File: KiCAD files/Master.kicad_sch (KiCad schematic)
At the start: 24 parts, among them SW1 EG1271A, SW2 EG1271A, SW3 EG1271A, SW4 EG1271A, U4 NUCLEO64-F446RE

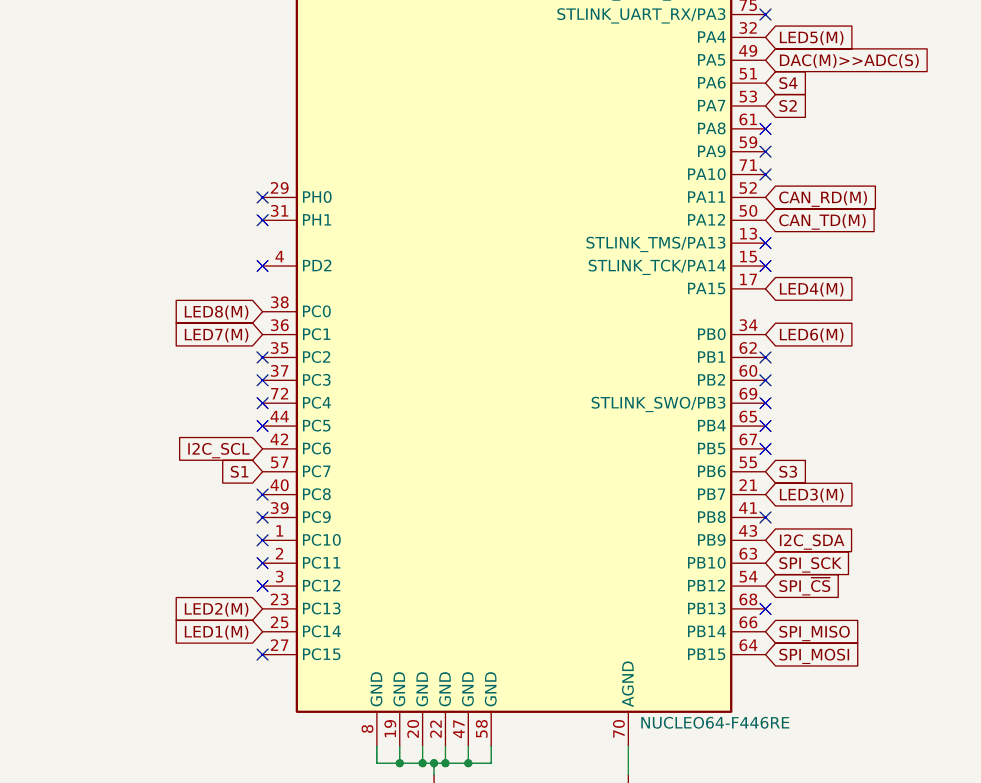
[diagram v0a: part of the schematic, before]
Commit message: update
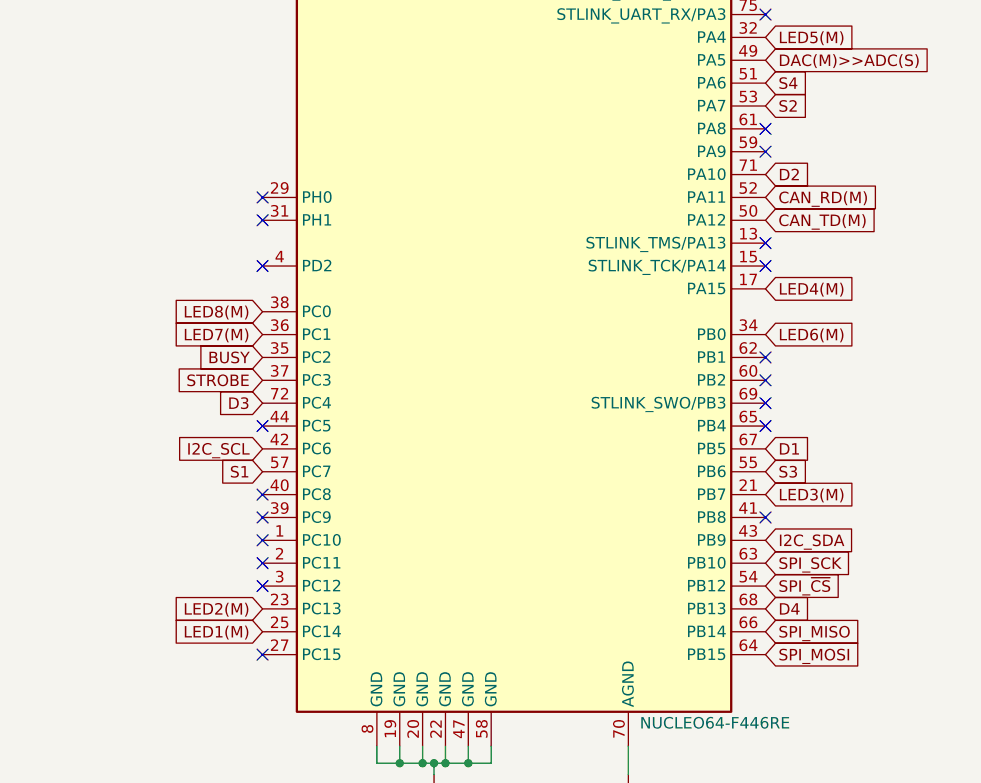
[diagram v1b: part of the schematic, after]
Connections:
- net BUSY: now reaches U4.35 (PC2)
- net STROBE: now reaches U4.37 (PC3)
- net D1: now reaches U4.67 (PB5)
- net D4: now reaches U4.68 (PB13)
- net D2: now reaches U4.71 (PA10)
- net D3: now reaches U4.72 (PC4)
- no-connect marks 40 -> 34
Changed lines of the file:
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@@
   )
   (no_connect (at 169.545 73.66))
-  (no_connect (at 113.665 101.6))
+  (no_connect (at 169.545 106.68))
   (no_connect (at 57.785 136.525))
   (no_connect (at 113.665 53.34))
-  (no_connect (at 169.545 76.2))
   (no_connect (at 113.665 116.84))
   (no_connect (at 113.665 106.68))
@@
   (no_connect (at 169.545 116.84))
   (no_connect (at 113.665 83.82))
-  (no_connect (at 113.665 99.06))
-  (no_connect (at 113.665 104.14))
   (no_connect (at 169.545 88.9))
   (no_connect (at 57.785 147.32))
@@
   (no_connect (at 169.545 104.14))
   (no_connect (at 139.065 40.64))
-  (no_connect (at 169.545 106.68))
   (no_connect (at 58.42 125.73))
   (no_connect (at 169.545 60.96))
@@
   (no_connect (at 144.145 40.64))
   (no_connect (at 131.445 40.64))
-  (no_connect (at 169.545 78.74))
   (no_connect (at 169.545 101.6))
   (no_connect (at 169.545 58.42))
@@
   (no_connect (at 128.905 40.64))
   (no_connect (at 113.665 88.9))
-  (no_connect (at 169.545 127))
+  (no_connect (at 169.545 99.06))
   (no_connect (at 113.665 132.08))
-  (no_connect (at 169.545 99.06))
+  (no_connect (at 169.545 76.2))
   (no_connect (at 126.365 40.64))
   (no_connect (at 169.545 86.36))
   (no_connect (at 113.665 114.3))
-  (no_connect (at 169.545 109.22))
   (no_connect (at 141.605 40.64))
   (wire (pts (xy 39.37 43.18) (xy 39.37 43.815))
@@
     )
   )
+  (global_label "D4" (shape input) (at 169.545 127 0) (fields_autoplaced)
+    (effects (font (size 1.27 1.27)) (justify left))
+    (property "Intersheetrefs" "${INTERSHEET_REFS}" (at 175.0097 127 0)
+      (effects (font (size 1.27 1.27)) (justify left) hide)
+    )
+  )
   (global_label "SPI_MISO" (shape input) (at 140.97 168.91 270) (fields_autoplaced)
     (effects (font (size 1.27 1.27)) (justify right))
@@
     )
   )
+  (global_label "D2" (shape input) (at 169.545 78.74 0) (fields_autoplaced)
+    (effects (font (size 1.27 1.27)) (justify left))
+    (property "Intersheetrefs" "${INTERSHEET_REFS}" (at 175.0097 78.74 0)
+      (effects (font (size 1.27 1.27)) (justify left) hide)
+    )
+  )
   (global_label "LED2(M)" (shape input) (at 29.845 38.1 90) (fields_autoplaced)
     (effects (font (size 1.27 1.27)) (justify left))
@@
     )
   )
+  (global_label "D3" (shape input) (at 113.665 104.14 180) (fields_autoplaced)
+    (effects (font (size 1.27 1.27)) (justify right))
+    (property "Intersheetrefs" "${INTERSHEET_REFS}" (at 108.2003 104.14 0)
+      (effects (font (size 1.27 1.27)) (justify right) hide)
+    )
+  )
   (global_label "S2" (shape input) (at 169.545 71.12 0) (fields_autoplaced)
     (effects (font (size 1.27 1.27)) (justify left))
@@
     )
   )
+  (global_label "STROBE" (shape input) (at 113.665 101.6 180) (fields_autoplaced)
+    (effects (font (size 1.27 1.27)) (justify right))
+    (property "Intersheetrefs" "${INTERSHEET_REFS}" (at 103.4832 101.6 0)
+      (effects (font (size 1.27 1.27)) (justify right) hide)
+    )
+  )
   (global_label "CAN_TD(M)" (shape input) (at 169.545 83.82 0) (fields_autoplaced)
     (effects (font (size 1.27 1.27)) (justify left))
@@
     )
   )
+  (global_label "BUSY" (shape input) (at 113.665 99.06 180) (fields_autoplaced)
+    (effects (font (size 1.27 1.27)) (justify right))
+    (property "Intersheetrefs" "${INTERSHEET_REFS}" (at 105.7812 99.06 0)
+      (effects (font (size 1.27 1.27)) (justify right) hide)
+    )
+  )
   (global_label "LED1(M)" (shape input) (at 20.32 38.1 90) (fields_autoplaced)
     (effects (font (size 1.27 1.27)) (justify left))
@@
       (effects (font (size 1.27 1.27)) (justify left) hide)
     )
+  )
+  (global_label "D1" (shape input) (at 169.545 109.22 0) (fields_autoplaced)
+    (effects (font (size 1.27 1.27)) (justify left))
+    (property "Intersheetrefs" "${INTERSHEET_REFS}" (at 175.0097 109.22 0)
+      (effects (font (size 1.27 1.27)) (justify left) hide)
+    )

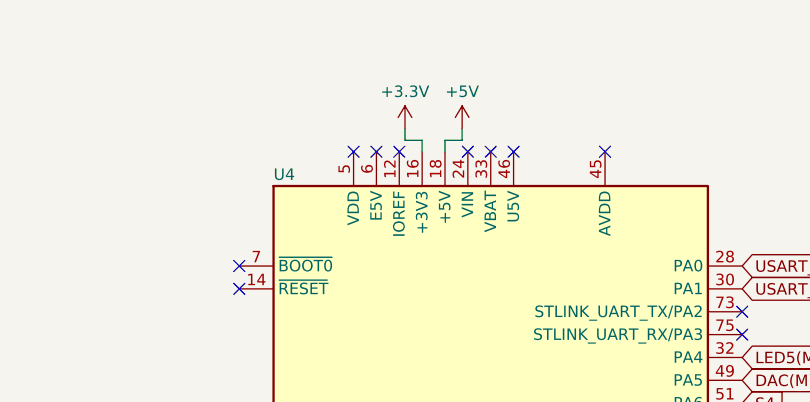
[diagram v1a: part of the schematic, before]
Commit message: update
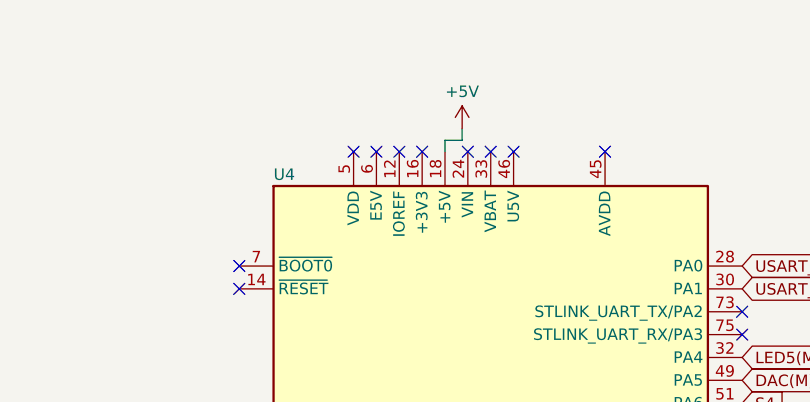
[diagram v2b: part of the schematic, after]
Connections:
- net +3.3V: no longer names the net of U4.16 (+3V3)
- no-connect marks 34 -> 35
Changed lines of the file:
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@@
   (no_connect (at 131.445 40.64))
   (no_connect (at 169.545 101.6))
+  (no_connect (at 133.985 40.64))
   (no_connect (at 169.545 58.42))
   (no_connect (at 113.665 119.38))
@@
     (stroke (width 0) (type default))
   )
-  (wire (pts (xy 133.985 39.37) (xy 132.08 39.37))
-    (stroke (width 0) (type default))
-  )
   (wire (pts (xy 20.955 82.55) (xy 20.955 84.455))
     (stroke (width 0) (type default))
@@
     (stroke (width 0) (type default))
   )
-  (wire (pts (xy 133.985 40.64) (xy 133.985 39.37))
-    (stroke (width 0) (type default))
-  )
   (wire (pts (xy 39.37 49.53) (xy 48.895 49.53))
     (stroke (width 0) (type default))
@@
   )
   (wire (pts (xy 136.525 39.37) (xy 138.43 39.37))
-    (stroke (width 0) (type default))
-  )
-  (wire (pts (xy 132.08 39.37) (xy 132.08 38.1))
     (stroke (width 0) (type default))
   )
@@
         )
       )
-    )
-  )
-  (symbol (lib_id "power:+3.3V") (at 132.08 38.1 0) (unit 1)
-    (in_bom yes) (on_board yes) (dnp no) (fields_autoplaced)
-    (property "Reference" "#PWR03" (at 132.08 41.91 0)
-      (effects (font (size 1.27 1.27)) hide)
-    )
-    (property "Value" "+3.3V" (at 132.08 33.9669 0)
-      (effects (font (size 1.27 1.27)))
-    )
-    (property "Footprint" "" (at 132.08 38.1 0)
-      (effects (font (size 1.27 1.27)) hide)
-    )
-    (property "Datasheet" "" (at 132.08 38.1 0)
-      (effects (font (size 1.27 1.27)) hide)
-    )
-    (pin "1")
-    (instances
-      (project "TVZ_KTM_ApplicationBoard"
-        (path "/e6e1ba2c-0a46-4bca-b3ad-33e778ea698b/7b36bbe9-69d8-437c-a840-f4b4d6c93da6"
-          (reference "#PWR03") (unit 1)
-        )
-      )
